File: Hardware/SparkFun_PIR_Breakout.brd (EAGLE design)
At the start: 12.7 x 16.5 mm, 18 parts, among them U1 EKMC4607112k

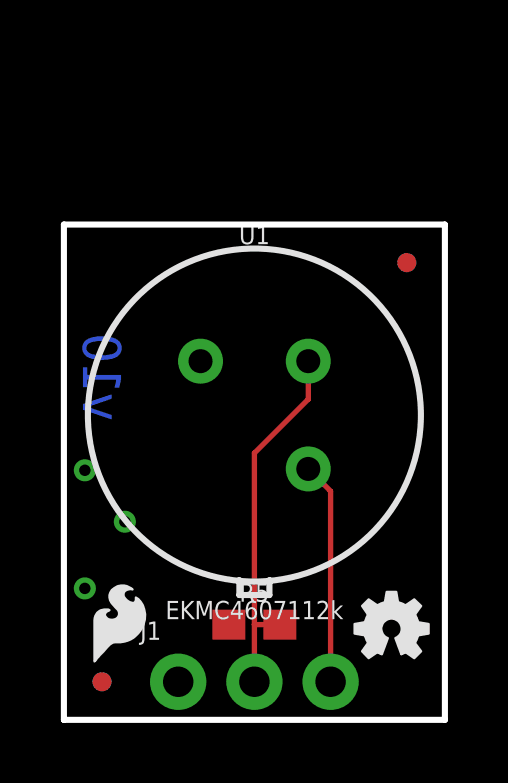
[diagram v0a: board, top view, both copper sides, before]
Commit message: post checklist changes
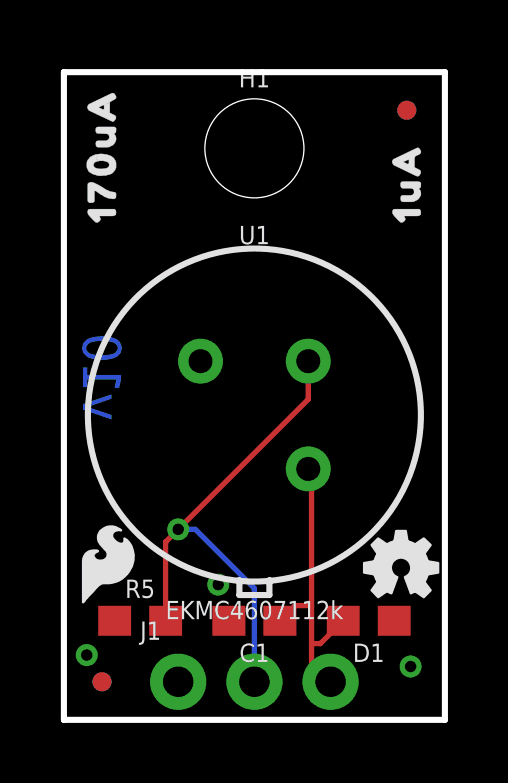
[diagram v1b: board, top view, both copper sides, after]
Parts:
- removed U$7: (no value), Labels-0_04:3.3V
- removed U$8: (no value), Labels-0_04:GND
- added C1: 0.1uF, SparkFun-Capacitors:0603
- added D1: 24V, SparkFun-DiscreteSemi:0603
- added H1: STAND-OFF, SparkFun-Hardware:STAND-OFF
- added U$1: (no value), output:#3V3#0
- added U$14: (no value), output:X0
- added U$16: (no value), output:Y0
- added U$3: (no value), output:#GND#0
- LOGO3: value SFE_LOGO_NAME.1_INCH -> SFE_LOGO_NAME_FLAME.1_INCH; device SparkFun-Aesthetics:SFE_LOGO_NAME_.1 -> SparkFun-Aesthetics:SFE_LOGO_NAME_FLAME_.1
- moved U$9 10.1 mm to (11.4, 15.9), flipped to the top, turned to 90 degrees
- moved U$2 9.00 mm to (1.27, 15.9), flipped to the top, turned to 90 degrees
- moved JP2 5.08 mm to (11.4, 20.3)
- moved JP9 5.08 mm to (11.4, 20.3)
- moved R5 3.81 mm to (2.54, 3.30)
- moved LOGO1 2.06 mm to (11.2, 5.08)
- moved LOGO4 2.01 mm to (1.46, 5.21)
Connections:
- net 3.3V: now also C1.1, D1.2
- net GND: now also C1.2, D1.1
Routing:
- net PIR_OUT: track 12.3 -> 18.0 mm, vias 0 -> 1
- net 3.3V: track 7.40 -> 10.0 mm
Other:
- board size 12.7 x 16.5 mm -> 12.7 x 21.6 mm

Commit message: checklist saved changes
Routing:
- net PIR_OUT: track 18.0 -> 17.1 mm
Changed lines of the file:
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@@
 <rectangle x1="0.762" y1="15.3035" x2="1.8415" y2="16.383" layer="31" rot="R90"/>
 <dimension x1="12.7" y1="0" x2="12.7" y2="21.59" x3="17.78" y3="10.795" textsize="1.778" layer="47" unit="inch"/>
-<dimension x1="12.7" y1="17.78" x2="0" y2="17.78" x3="6.35" y3="24.13" textsize="1.778" layer="47" unit="inch"/>
+<dimension x1="12.7" y1="17.78" x2="0" y2="17.78" x3="6.35" y3="26.67" textsize="1.778" layer="47" unit="inch"/>
 <wire x1="10.9855" y1="7.747" x2="9.7155" y2="7.747" width="0.254" layer="22"/>
 <wire x1="9.7155" y1="7.747" x2="10.033" y2="7.4295" width="0.254" layer="22"/>
@@
 <wire x1="12.0015" y1="10.668" x2="11.684" y2="10.3505" width="0.254" layer="22"/>
 <wire x1="12.0015" y1="10.668" x2="12.319" y2="10.3505" width="0.254" layer="22"/>
+<dimension x1="6.35" y1="19.05" x2="0" y2="19.05" x3="3.175" y3="22.86" textsize="1.778" layer="47" unit="inch"/>
+<dimension x1="6.35" y1="19.05" x2="6.35" y2="0" x3="-3.81" y3="9.525" textsize="1.778" layer="47" unit="inch"/>
 </plain>
 <attributes>
@@
 <wire x1="8.146" y1="10.686" x2="3.81" y2="6.35" width="0.1778" layer="1"/>
 <wire x1="3.81" y1="6.35" x2="3.39" y2="5.93" width="0.1778" layer="1"/>
-<wire x1="3.39" y1="3.302" x2="3.67475" y2="3.302" width="0.1778" layer="1"/>
-<wire x1="5.70675" y1="1.27" x2="6.35" y2="1.27" width="0.1778" layer="1"/>
 <wire x1="6.35" y1="1.27" x2="6.35" y2="4.3815" width="0.1778" layer="16"/>
 <wire x1="6.35" y1="4.3815" x2="4.3815" y2="6.35" width="0.1778" layer="16"/>
@@
 <mfgpreviewcolor name="substratecolor" color="0xFF786E46"/>
 </mfgpreviewcolors>
-<errors>
-</errors>
 </board>
 </drawing>
